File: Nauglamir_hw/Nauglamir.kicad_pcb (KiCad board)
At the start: 4 copper layers, 54.6 x 54.6 mm, 69 parts, among them Q1 2N7002

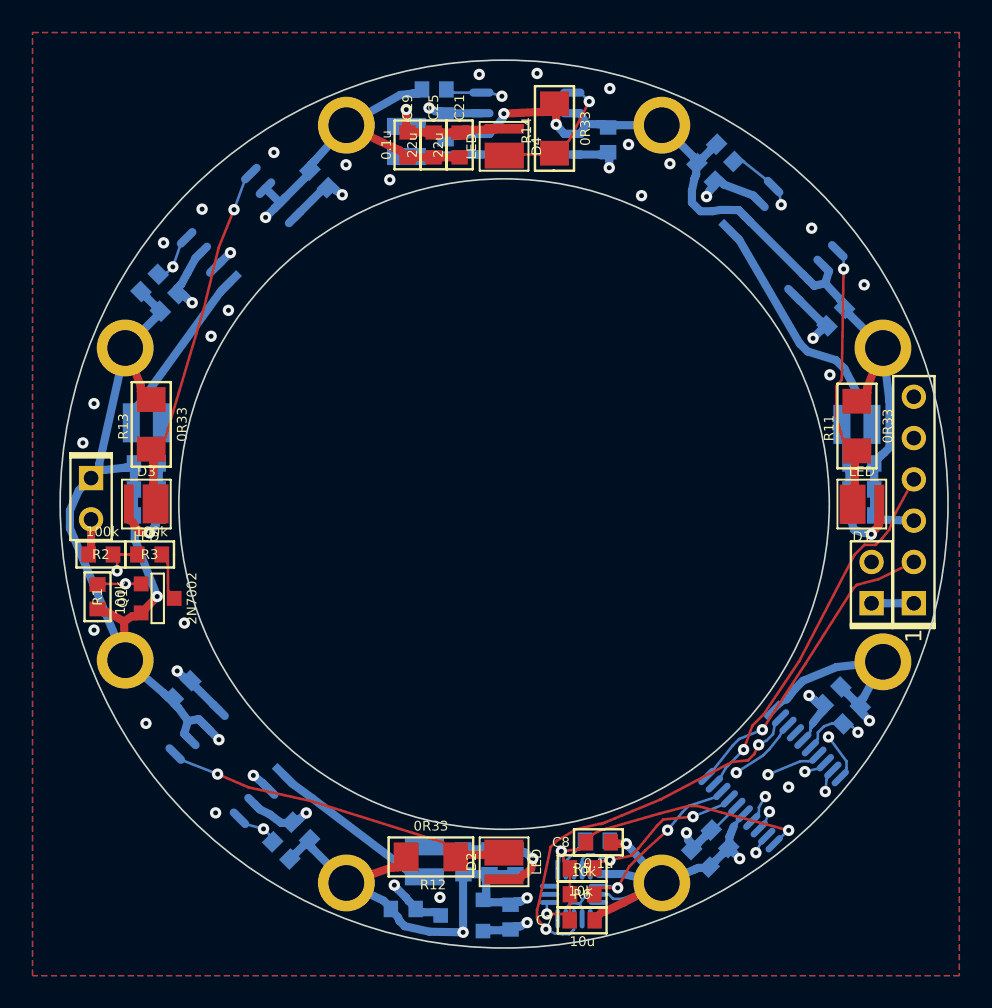
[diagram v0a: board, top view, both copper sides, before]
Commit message: Routed
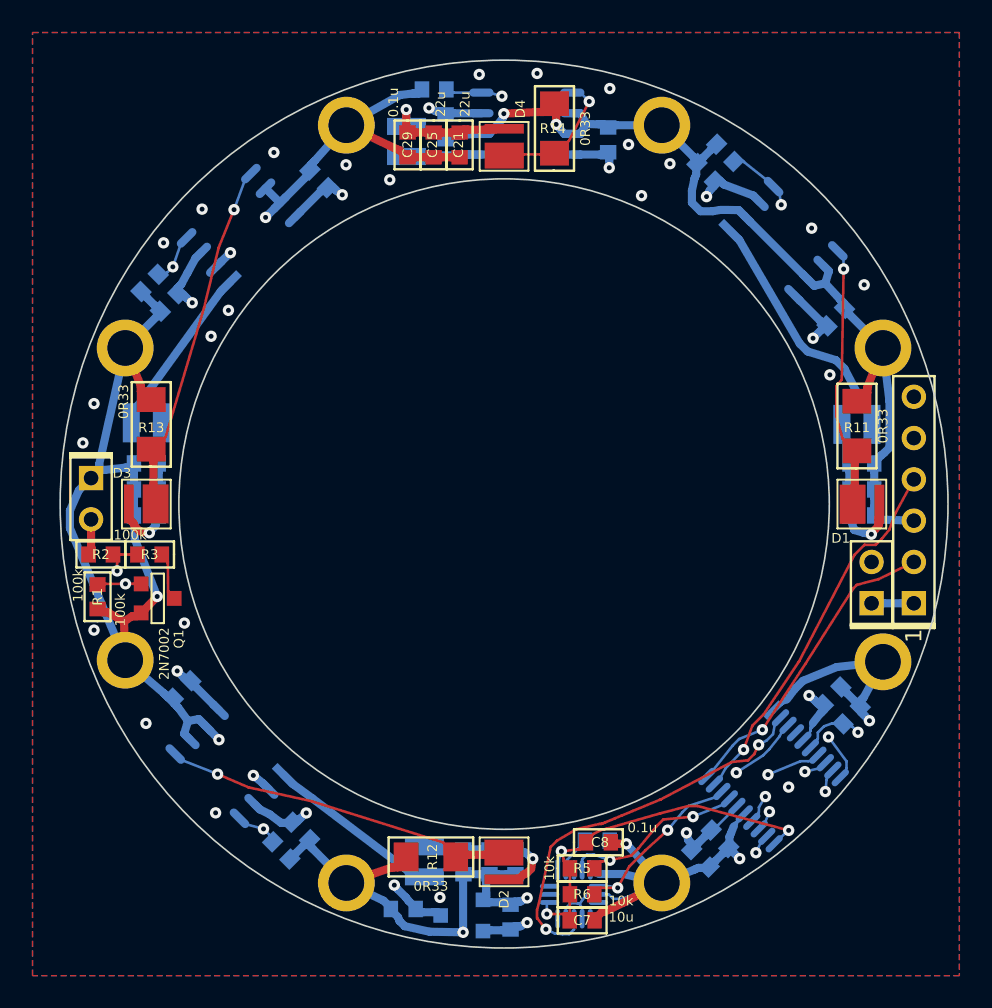
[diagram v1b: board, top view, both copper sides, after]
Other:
- rule pad_to_mask_clearance: 0 -> 0.06
